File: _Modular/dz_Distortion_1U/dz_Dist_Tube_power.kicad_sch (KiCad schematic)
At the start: 65 parts, among them J1 Unreg +20..24v, J2 AC +20..24v, J3 Heater 6,3v, J4 Heater 6,3v, J5 Anode +300v, Q1 BD140, Q2 BD139, Q3 IRF4905, Q4 IRF4905, Q5 KT3107, Q6 IRF830, U1 TL494, U2 MC34063AP

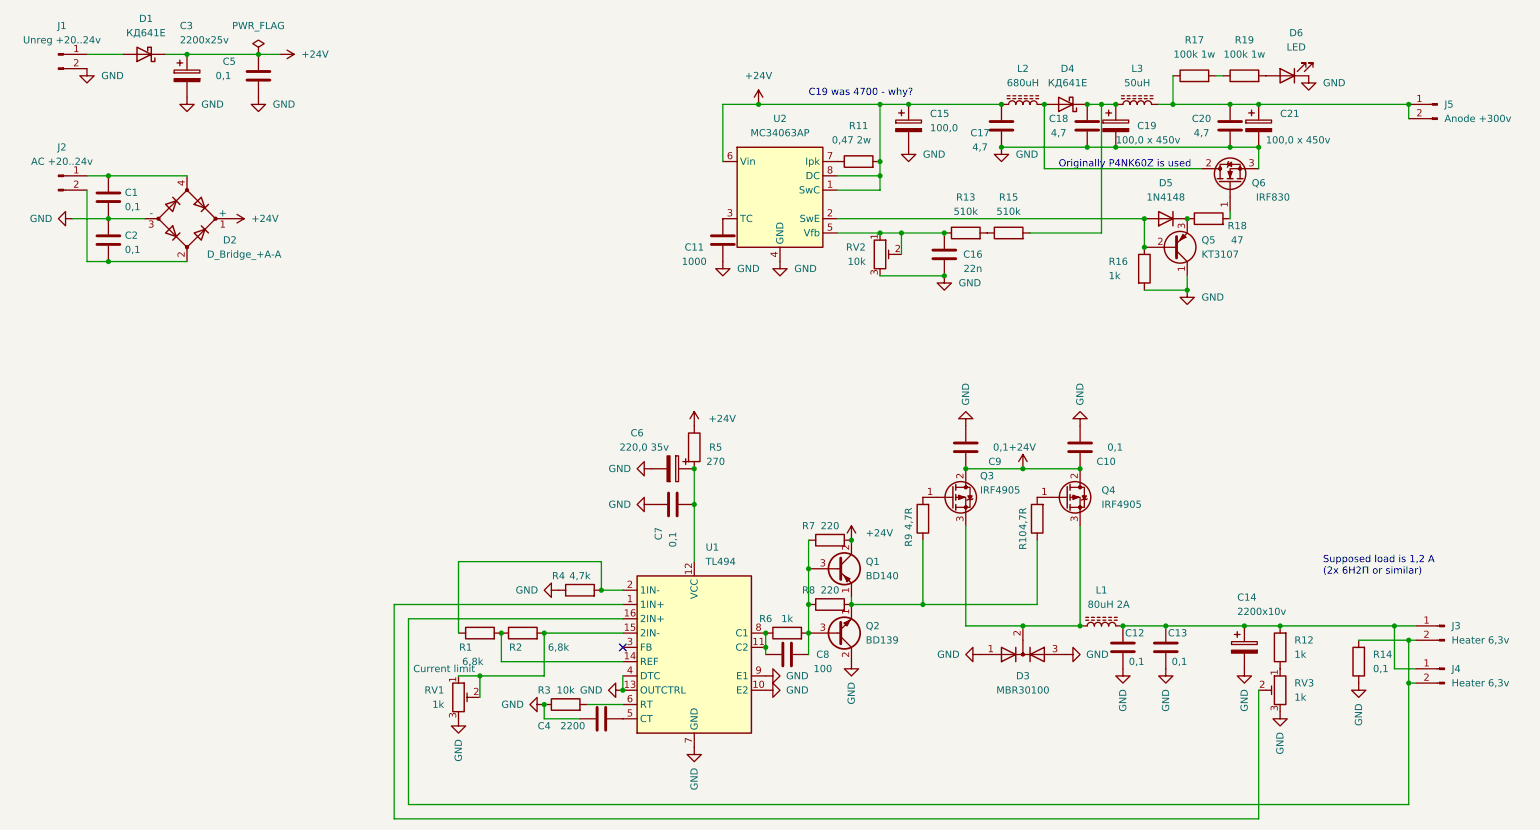
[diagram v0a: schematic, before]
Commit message: up
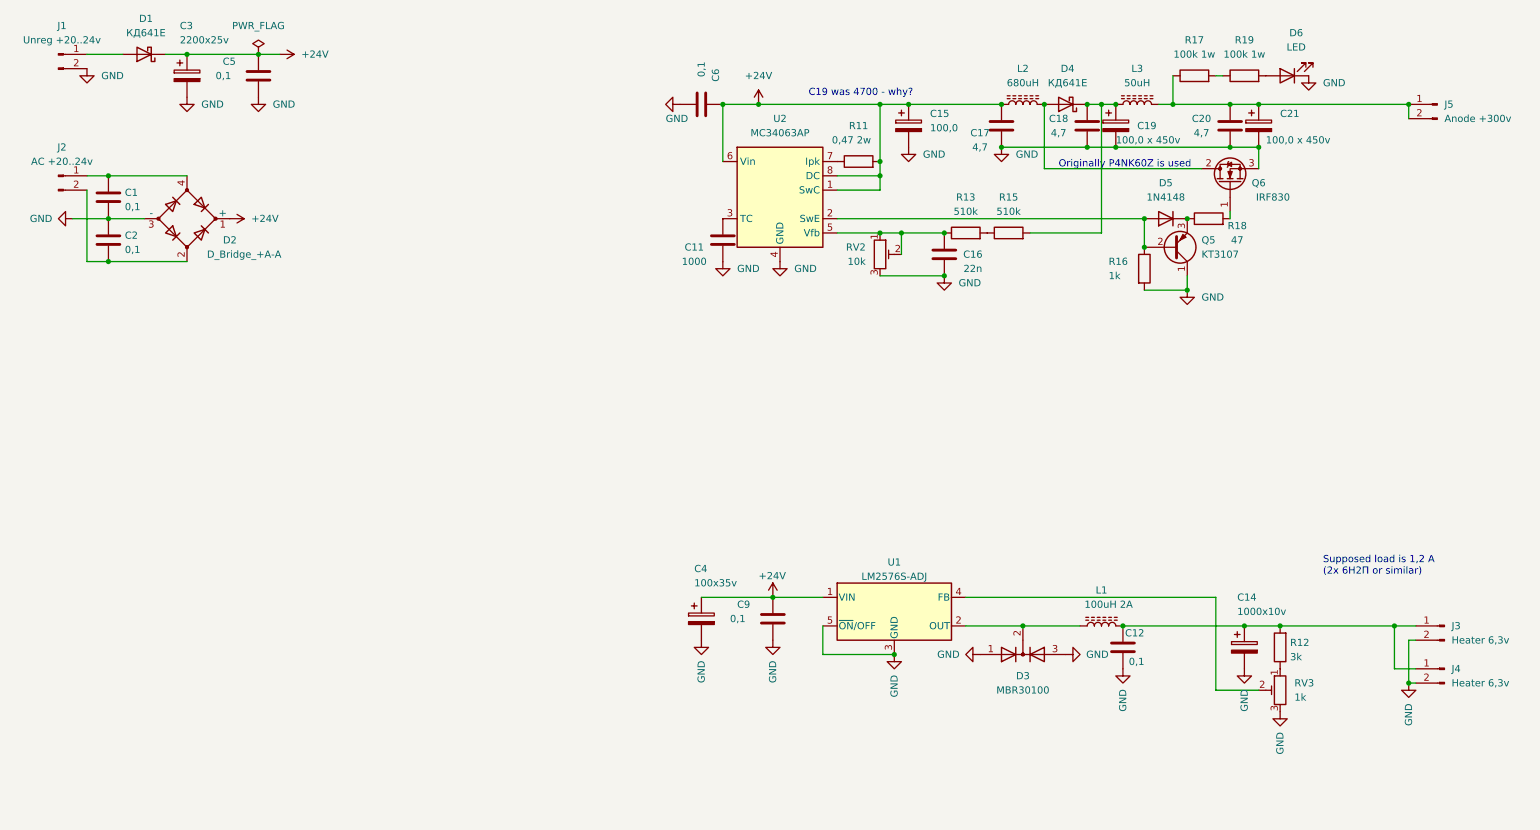
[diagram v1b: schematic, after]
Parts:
- removed C10, C13, C7: 0,1, Capacitor_SMD:C_1206_3216Metric_Pad1.33x1.80mm_HandSolder, symbol Device:C
- removed C4: 2200, Capacitor_SMD:C_0805_2012Metric_Pad1.18x1.45mm_HandSolder, symbol Device:C
- removed C6: 220,0 35v, Capacitor_THT:CP_Radial_D8.0mm_P2.50mm, symbol Device:C_Polarized
- removed C8: 100, Capacitor_SMD:C_0805_2012Metric_Pad1.18x1.45mm_HandSolder, symbol Device:C
- removed Q1: BD140, Package_TO_SOT_THT:TO-126-3_Vertical, symbol Transistor_BJT:BD140
- removed Q2: BD139, Package_TO_SOT_THT:TO-126-3_Vertical, symbol Transistor_BJT:BD139
- removed Q3, Q4: IRF4905, Package_TO_SOT_THT:TO-220-3_Vertical, symbol Transistor_FET:IRF4905
- removed R1, R2: 6,8k, Resistor_SMD:R_1206_3216Metric_Pad1.30x1.75mm_HandSolder, symbol Device:R
- removed R10, R9: 4,7R, Resistor_THT:R_Axial_DIN0414_L11.9mm_D4.5mm_P5.08mm_Vertical, symbol Device:R
- removed R14: 0,1, Resistor_THT:R_Axial_DIN0414_L11.9mm_D4.5mm_P5.08mm_Vertical, symbol Device:R
- removed R3: 10k, Resistor_SMD:R_1206_3216Metric_Pad1.30x1.75mm_HandSolder, symbol Device:R
- removed R4: 4,7k, Resistor_SMD:R_1206_3216Metric_Pad1.30x1.75mm_HandSolder, symbol Device:R
- removed R5: 270, Resistor_SMD:R_1206_3216Metric_Pad1.30x1.75mm_HandSolder, symbol Device:R
- removed R6: 1k, Resistor_SMD:R_1206_3216Metric_Pad1.30x1.75mm_HandSolder, symbol Device:R
- removed R7, R8: 220, Resistor_SMD:R_1206_3216Metric_Pad1.30x1.75mm_HandSolder, symbol Device:R
- removed RV1: 1k, Resistor_SMD:R_1206_3216Metric_Pad1.30x1.75mm_HandSolder, symbol Device:R_Potentiometer_Trim
- removed U1: TL494, Package_DIP:DIP-16_W7.62mm_LongPads, symbol Regulator_Controller:TL494
- added C4: 100x35v, Capacitor_THT:CP_Radial_D10.0mm_P5.00mm, symbol Device:C_Polarized
- added C6: 0,1, Capacitor_SMD:C_1206_3216Metric_Pad1.33x1.80mm_HandSolder, symbol Device:C
- added U1: LM2576S-ADJ, Package_TO_SOT_SMD:TO-263-5_TabPin3, symbol Regulator_Switching:LM2576S-ADJ
- C14: value 2200x10v -> 1000x10v
- D5: footprint Diode_THT:D_DO-35_SOD27_P7.62mm_Horizontal -> Diode_THT:D_DO-35_SOD27_P2.54mm_Vertical_KathodeUp
- L1: value 80uH 2A -> 100uH 2A
- R11: footprint Resistor_THT:R_Axial_DIN0309_L9.0mm_D3.2mm_P12.70mm_Horizontal -> Resistor_THT:R_Axial_DIN0411_L9.9mm_D3.6mm_P5.08mm_Vertical
- R12: value 1k -> 3k
- RV3: footprint Resistor_SMD:R_1206_3216Metric_Pad1.30x1.75mm_HandSolder -> Potentiometer_THT:Potentiometer_Runtron_RM-065_Vertical
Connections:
- net +24V: now also C4.1, C6.1, U1.1 (VIN)
- net GND: now also J3.2 (Pin_2), J4.2 (Pin_2), C4.2, C6.2, U1.3 (GND), U1.5 (~{ON}/OFF)
- net at RV3.2: now also U1.4 (FB)
- net at D3.2 (K), L1.1: now also U1.2 (OUT)
- no-connect marks 1 -> 0
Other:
- moved on the sheet: C9

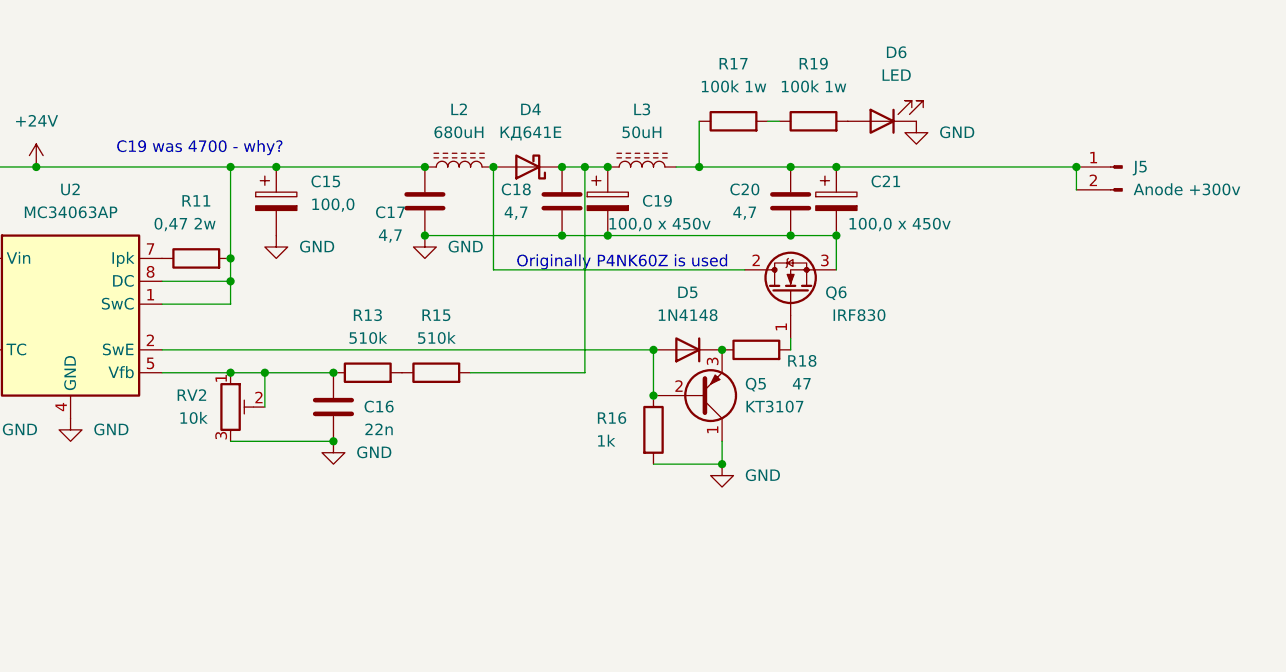
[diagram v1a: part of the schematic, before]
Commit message: up
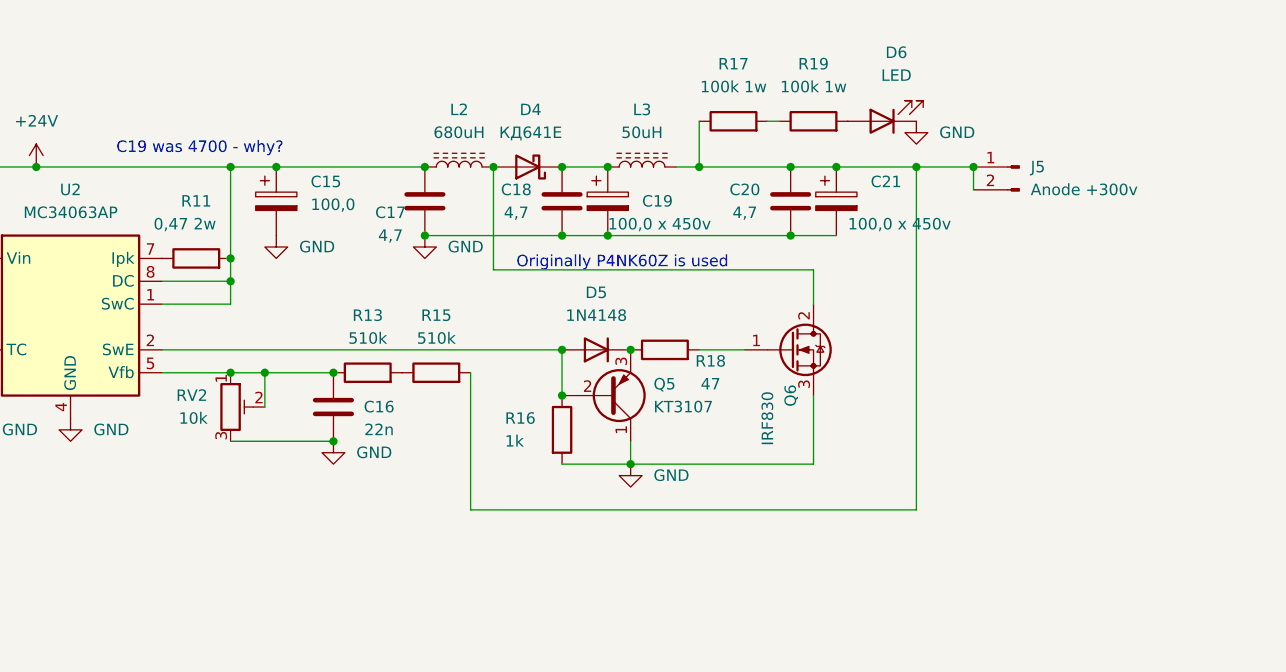
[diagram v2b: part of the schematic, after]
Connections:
- net at C18.2, C19.1, D4.1 (K)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: no longer R15.2
- net at C20.2, C21.1, J5.1 (Pin_1)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: now also R15.2
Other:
- moved on the sheet: D5, J5, Q5, Q6, R16, R18
